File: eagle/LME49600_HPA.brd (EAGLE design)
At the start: 93.7 x 71.1 mm, 47 parts, among them IC1 OPA2134P, IC2 OPA2134P, P1 POLYSWITCH, P2 POLYSWITCH

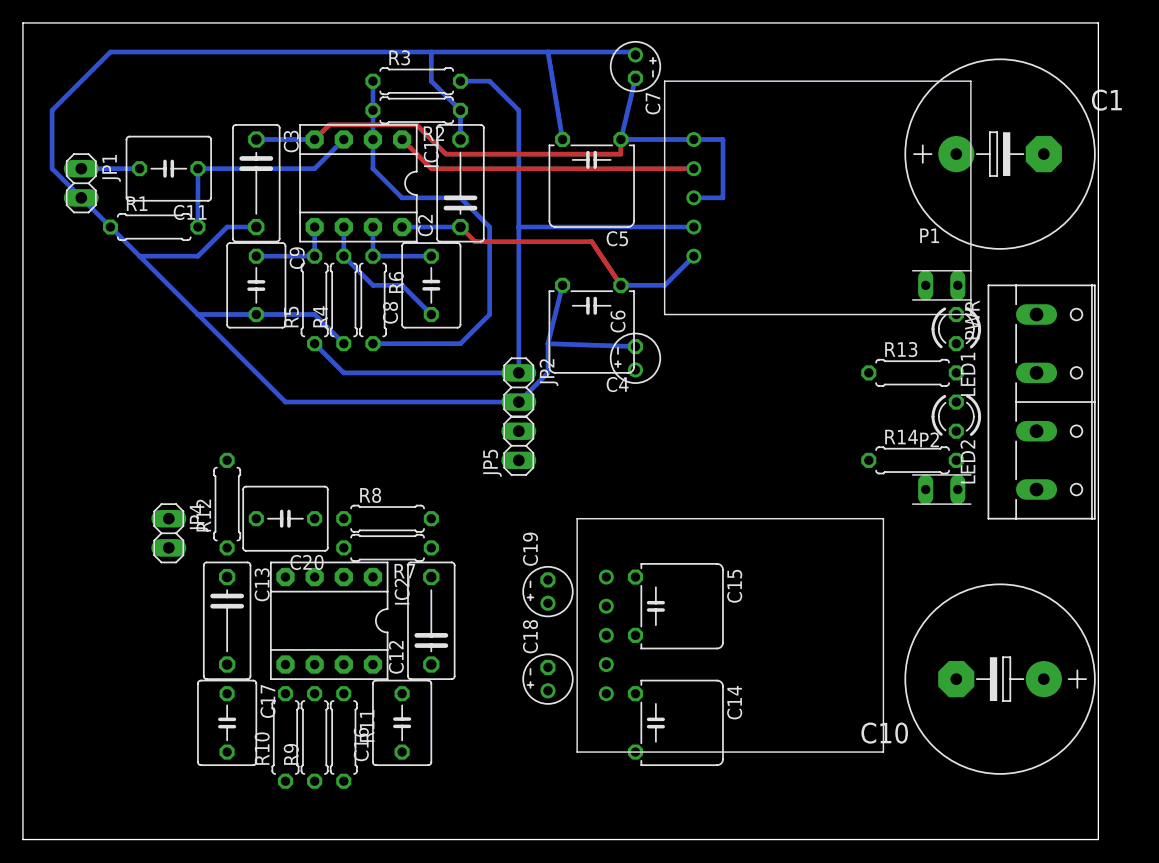
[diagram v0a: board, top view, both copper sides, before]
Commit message: Update: Board design
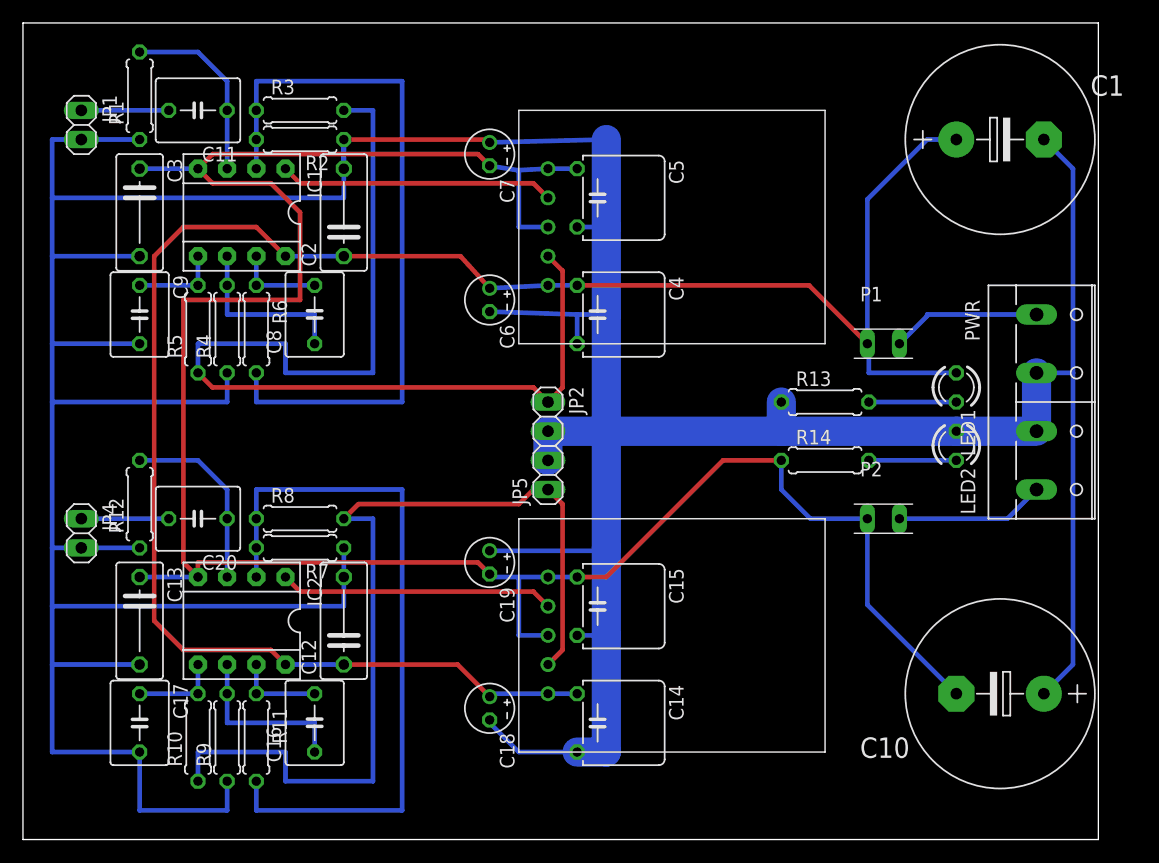
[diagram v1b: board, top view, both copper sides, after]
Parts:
- moved C7 14.8 mm to (40.6, 59.7)
- moved C6 13.7 mm to (40.6, 47.0), turned to 270 degrees
- moved U$1 13.0 mm to (53.3, 53.3)
- moved R1 11.5 mm to (10.2, 64.8), turned to 90 degrees
- moved C8 10.5 mm to (25.4, 45.7)
- moved C2 10.5 mm to (27.9, 54.6)
- moved C3 10.5 mm to (10.2, 54.6)
- moved C9 10.5 mm to (10.2, 45.7)
- moved IC1 10.5 mm to (19.1, 54.6)
- moved R2 10.5 mm to (24.1, 61.0)
- moved R3 10.5 mm to (24.1, 63.5)
- moved R4 10.5 mm to (17.8, 44.5)
- moved R6 10.5 mm to (20.3, 44.5)
- moved R5 10.5 mm to (15.2, 44.5)
- moved R13 8.03 mm to (69.8, 38.1)
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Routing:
- net AGND: track 167.5 -> 418.5 mm
- net V+: track 29.0 -> 171.7 mm
- net V-: track 56.6 -> 198.6 mm
- net N$13: track 0.00 -> 80.8 mm
- net N$4: track 0.00 -> 63.5 mm
- net N$14: track 63.1 -> 91.0 mm
- net N$3: track 38.7 -> 63.5 mm
- net N$5: track 0.00 -> 23.9 mm
- net N$16: track 0.00 -> 16.3 mm
- net N$9: track 0.00 -> 15.2 mm
- net PW+: track 0.00 -> 13.1 mm
- net PW-: track 0.00 -> 13.0 mm
- net N$19: track 0.00 -> 7.62 mm
- net N$17: track 0.00 -> 7.62 mm
- net N$10: track 0.00 -> 7.62 mm
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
